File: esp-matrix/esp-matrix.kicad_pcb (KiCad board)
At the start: 2 copper layers, 25.4 x 54.6 mm, 30 parts, among them P1 CONN_01X02, P2 CONN_01X02, SW1 SW_PUSH_SMALL, SW2 SW_PUSH_SMALL, U1 ESP-12E, U2 MCP1700-3.0, U3 SI7021, U4 BMP180

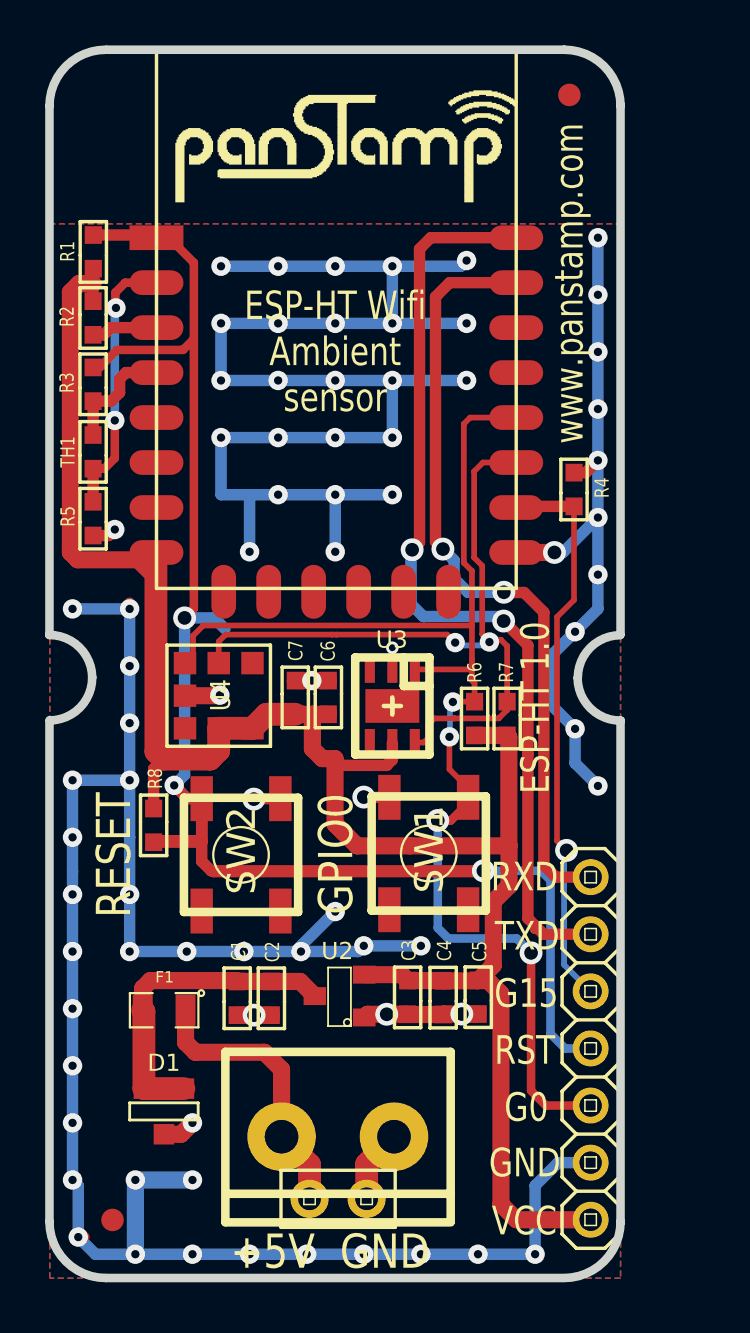
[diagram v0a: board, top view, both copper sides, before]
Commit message: First version finished
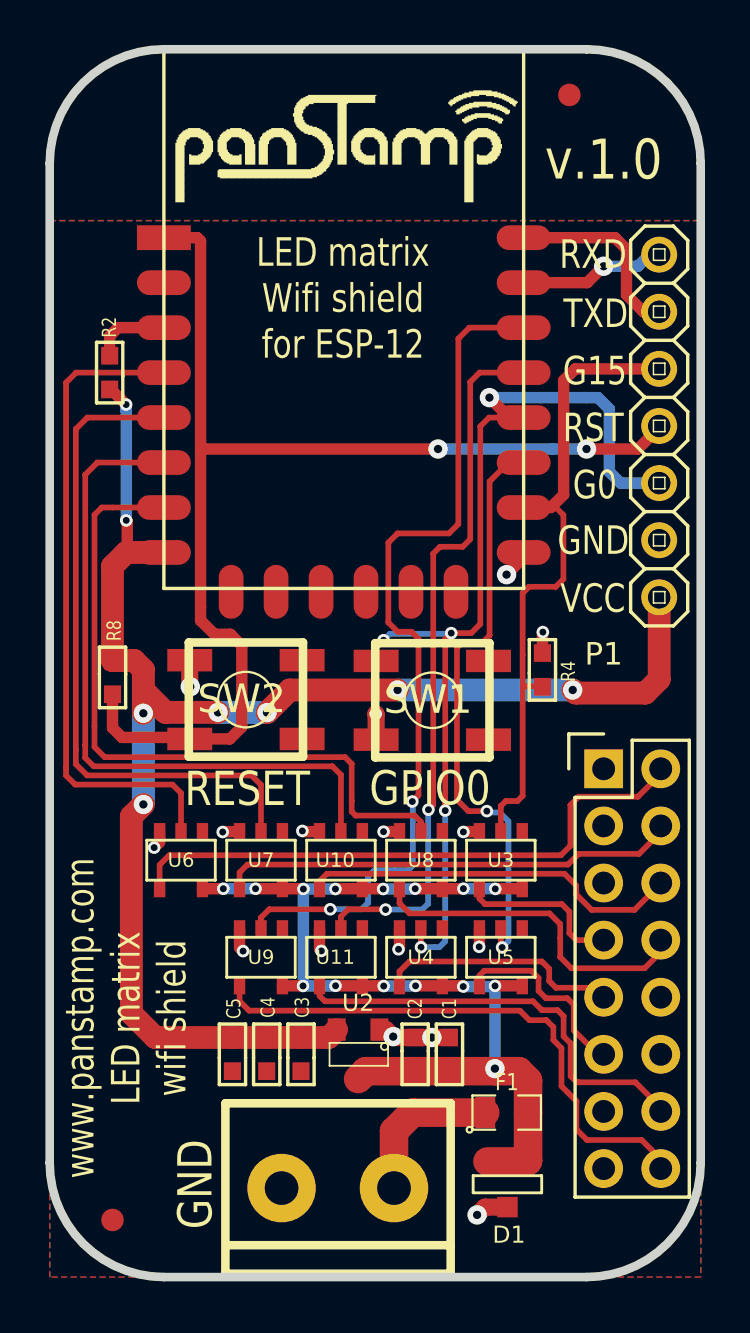
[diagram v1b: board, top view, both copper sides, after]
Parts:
- removed C6: 100n, SM0603S
- removed C7: 1u, mysmd:SM0603S
- removed the P2 at (148.7, 96.1)
- removed R1, R5, R6, R7: 10k, mysmd:SM0603S
- removed R3: 0, mysmd:SM0603S
- removed TH1: THERMISTOR, mysmd:SM0603S
- added P1: CONN_02X08, Pin_Headers:Pin_Header_Straight_2x08, F.Cu at (160.5, 77.0)
- added U10: 74AHC1G34, libcms:SOT23-5, F.Cu at (148.8, 81.0)
- added U11: 74AHC1G34, libcms:SOT23-5, F.Cu at (148.8, 85.3)
- added U5: 74AHC1G34, libcms:SOT23-5, F.Cu at (156.0, 85.3)
- added U6: 74AHC1G34, libcms:SOT23-5, F.Cu at (141.7, 81.0)
- added U7: 74AHC1G34, libcms:SOT23-5, F.Cu at (145.3, 81.0)
- added U8: 74AHC1G34, libcms:SOT23-5, F.Cu at (152.4, 81.0)
- added U9: 74AHC1G34, libcms:SOT23-5, F.Cu at (145.3, 85.3)
- U2: value MCP1700-3.0 -> MCP1702-3.3
- U3: value SI7021 -> 74AHC1G34; footprint mysmd:DFN-6 -> libcms:SOT23-5
- U4: value BMP180 -> 74AHC1G34; footprint mysmd:BMP180 -> libcms:SOT23-5
- moved PROG1 27.9 mm to (163.0, 61.7)
- moved F1 15.9 mm to (156.2, 92.3), turned to 0 degrees
- moved D1 15.6 mm to (156.2, 95.4)
- moved U4 14.7 mm to (152.4, 85.3), turned to 180 degrees
- moved C5 11.2 mm to (144.0, 89.7)
- moved C1 9.76 mm to (153.7, 89.7), turned to 90 degrees
- moved U3 8.39 mm to (156.0, 81.0)
- moved C4 8.24 mm to (145.5, 89.7)
- moved R4 8.14 mm to (157.8, 72.6)
- moved SW2 6.91 mm to (144.6, 73.9), turned to 0 degrees
- moved C2 6.86 mm to (152.1, 89.7), turned to 90 degrees
- moved R8 6.83 mm to (138.7, 72.9)
- moved SW1 6.82 mm to (152.9, 73.9), turned to 0 degrees
- moved C3 5.38 mm to (147.1, 89.7)
- moved U2 2.72 mm to (149.6, 89.7), turned to 180 degrees
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- renumbered P1 to P2
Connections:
- C1 pad 1: Net-(C1-Pad1) -> +5V
- C2 pad 1: Net-(C1-Pad1) -> +5V
- D1 pad 1: Net-(C1-Pad1) -> +5V
- D1 pad 2: Net-(C1-Pad1) -> +5V
- F1 pad 2: Net-(C1-Pad1) -> +5V
- P2 pad 1: Net-(F1-Pad1) -> GND
- P2 pad 2: GND -> Net-(F1-Pad1)
- U2 pad 3: Net-(C1-Pad1) -> +5V
- U3 pad 1: /GPIO0 -> (no net)
- U3 pad 2: GND -> /GPIO15
- U3 pad 3: (no net) -> GND
- U3 pad 4: (no net) -> /EN
- U3 pad 5: VCC -> +5V
- U4 pad 2: VCC -> /GPIO0
- U4 pad 3: VCC -> GND
- U4 pad 4: (no net) -> /R1
- U4 pad 5: /GPIO2 -> +5V
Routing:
- net GND: track 139.8 -> 17.1 mm, vias 53 -> 16
- net (no net): track 63.4 -> 0.00 mm, vias 24 -> 0
- net +5V: track 0.00 -> 46.6 mm, vias 0 -> 15
- net /GPIO5: track 0.00 -> 39.1 mm, vias 0 -> 2
- net /RESET: track 88.0 -> 53.1 mm, vias 3 -> 2
- net /TXD: track 41.9 -> 8.58 mm, vias 2 -> 0
- net /GPIO4: track 0.00 -> 31.8 mm, vias 0 -> 2
- net /GPIO13: track 0.00 -> 31.1 mm
- net /GPIO12: track 0.00 -> 30.5 mm
- net /GPIO14: track 0.00 -> 29.7 mm
- net VCC: track 98.2 -> 68.8 mm, vias 0 -> 8
- net /RXD: track 34.9 -> 6.54 mm, vias 2 -> 1
- net /LA: track 0.00 -> 26.3 mm
- net /SK: track 0.00 -> 24.8 mm
- net /GPIO16: track 5.21 -> 29.2 mm
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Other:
- board size 25.4 x 54.6 mm -> 29 x 54.6 mm
- board text added: "LED matrix Wifi shield for ESP-12"
- board text added: "v.1.0"
- board text added: "www.panstamp.com LED matrix wifi shield"
- board text removed: "+5V GND"
- board text removed: "ESP-HT 1.0"
- board text removed: "ESP-HT Wifi Ambient sensor"
- board text removed: "www.panstamp.com"
